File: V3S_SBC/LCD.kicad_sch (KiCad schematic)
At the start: 2 parts, among them J4 Conn_01x40_Pin, J5 Conn_01x06_Pin

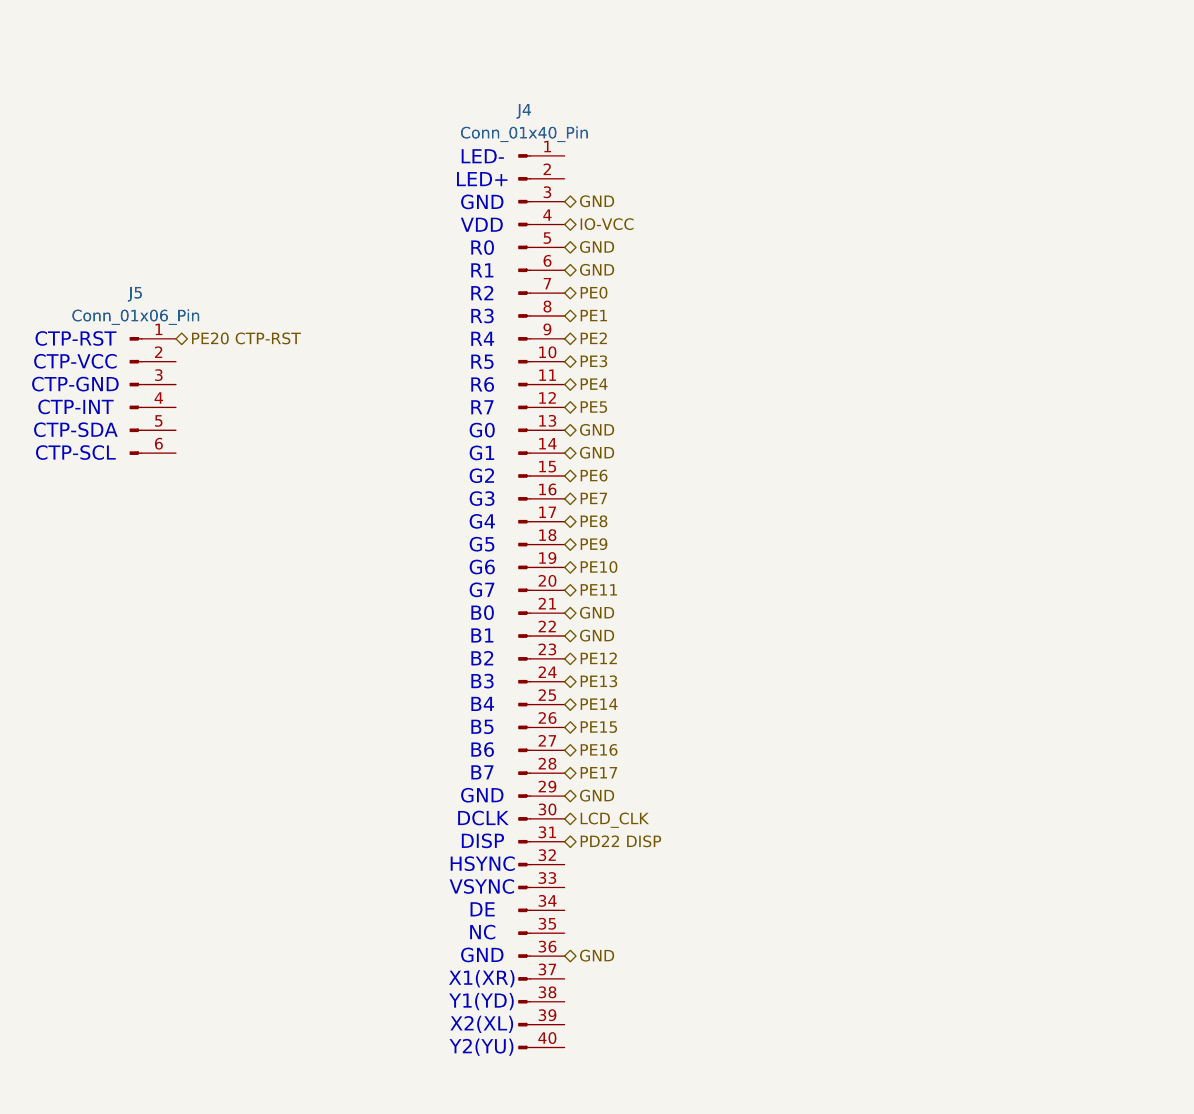
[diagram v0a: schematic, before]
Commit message: Add files via upload
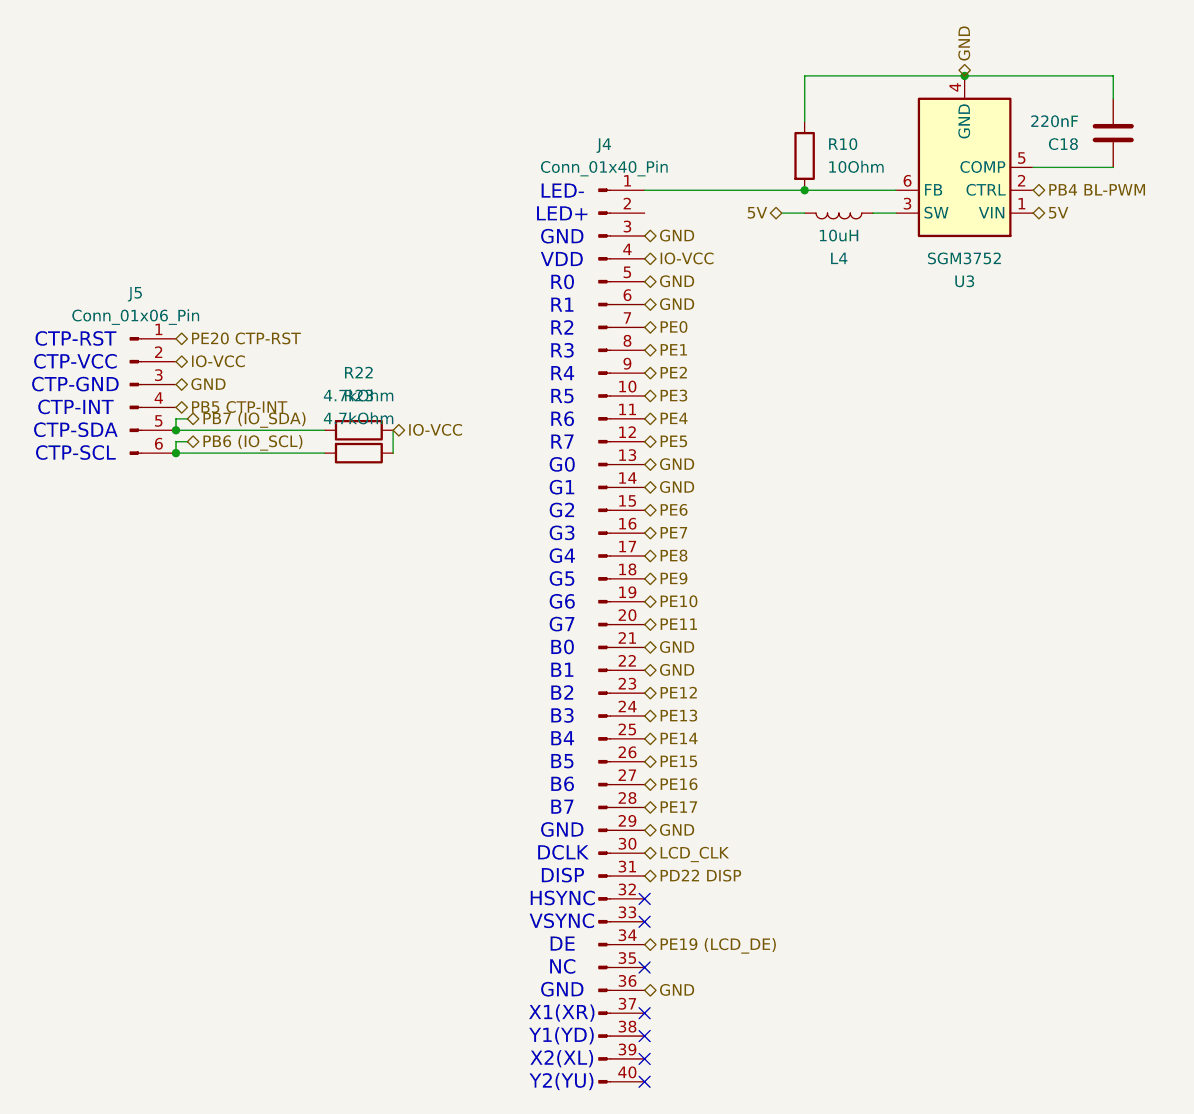
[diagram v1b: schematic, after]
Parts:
- added C18: 220nF, symbol Device:C
- added L4: 10uH, symbol Device:L
- added R10: 10Ohm, symbol Device:R
- added R22, R23: 4.7kOhm, symbol Device:R
- added U3: SGM3752, Package_TO_SOT_SMD:SOT-23-6, symbol Driver_LED:TPS61165DBV
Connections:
- net GND: now also J5.3 (Pin_3), C18.2, R10.1, U3.4 (GND)
- net IO-VCC: now also J5.2 (Pin_2), R22.1, R23.1
- net PB5 CTP-INT: now reaches J5.4 (Pin_4)
- net PB7 (IO_SDA): now reaches J5.5 (Pin_5)
- net PB7 (IO_SDA): now also R22.2
- net PB6 (IO_SCL): now reaches J5.6 (Pin_6)
- net PB6 (IO_SCL): now also R23.2
- net at J4.1 (Pin_1): now also R10.2, U3.6 (FB)
- net PE19 (LCD_DE): now reaches J4.34 (Pin_34)
- new net: L4.1, U3.3 (SW)
- new net: C18.1, U3.5 (COMP)
- new net 5V: L4.2, U3.1 (VIN)
- new net PB4 BL-PWM: U3.2 (CTRL)
- no-connect marks 0 -> 7
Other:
- moved on the sheet: J4
